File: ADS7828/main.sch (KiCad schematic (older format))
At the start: 12 parts, among them P1 Analog input connector, P2 Address 0, P3 Address 1, P4 I2C Connector, P5 Power Connector, U1 ADS7828

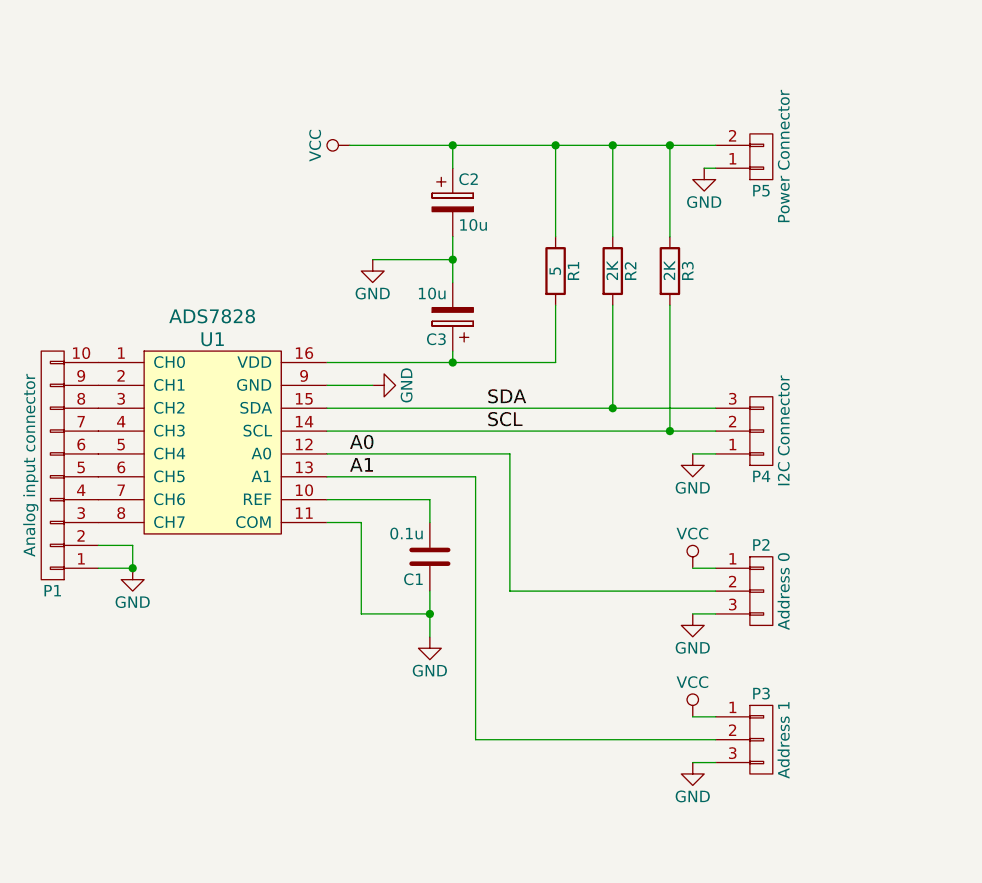
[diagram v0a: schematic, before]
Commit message: test
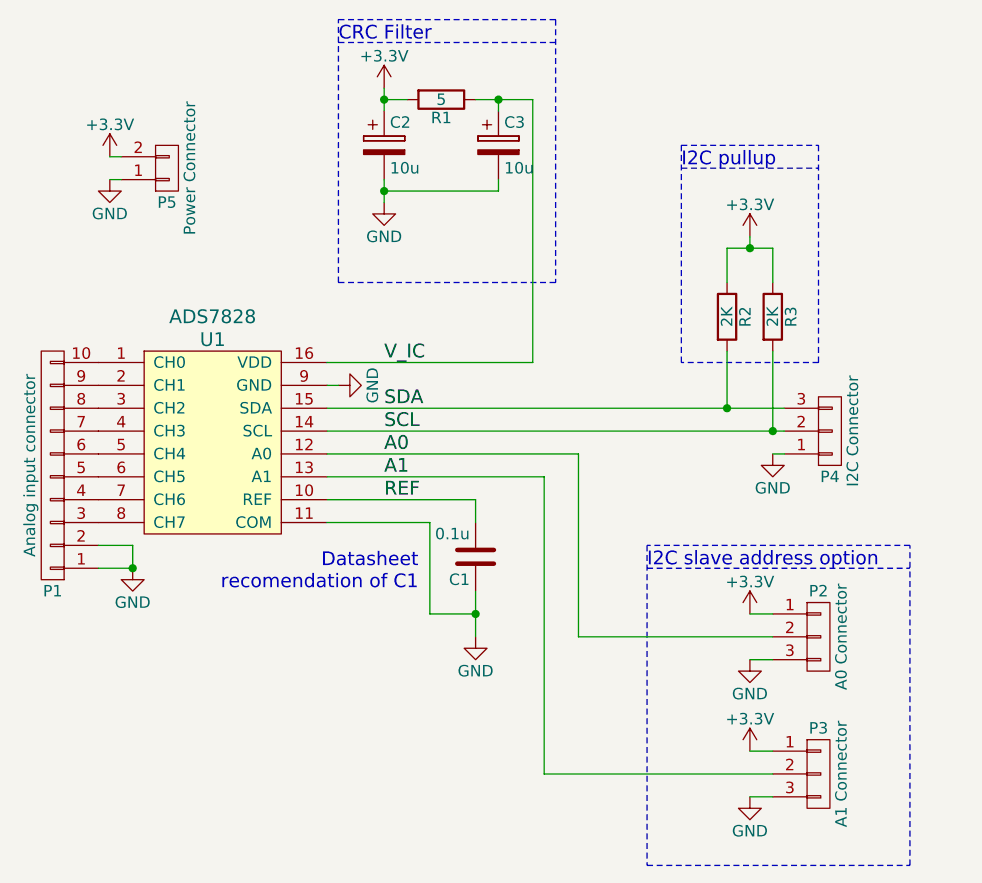
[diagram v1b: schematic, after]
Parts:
- P2: value Address 0 -> A0 Connector
- P3: value Address 1 -> A1 Connector
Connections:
- net REF: now reaches C1.2, U1.10 (REF)
- net V_IC: now reaches C3.1, U1.16 (VDD)
- net V_IC: now also R1.1; no longer R1.2
- net VCC renamed +3V3
- net +3V3: now also R1.2; no longer R1.1
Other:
- note added: "CRC Filter"
- note added: "Datasheet \nrecomendation of C1"
- note added: "I2C pullup"
- note added: "I2C slave address option"
- moved on the sheet: C1, C2, C3, P2, P3, P4, P5, R1, R2, R3
